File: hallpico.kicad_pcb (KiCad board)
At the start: 2 copper layers, 61 x 58.4 mm, 20 parts, among them J1 BOOT Jump Wire, SW1 SW_SPST, SW2 SW_SPST, U1 RP2040 MiniPico V1.1, U2 GH39FKSW, U3 GH39FKSW, U4 GH39FKSW, U5 GH39FKSW

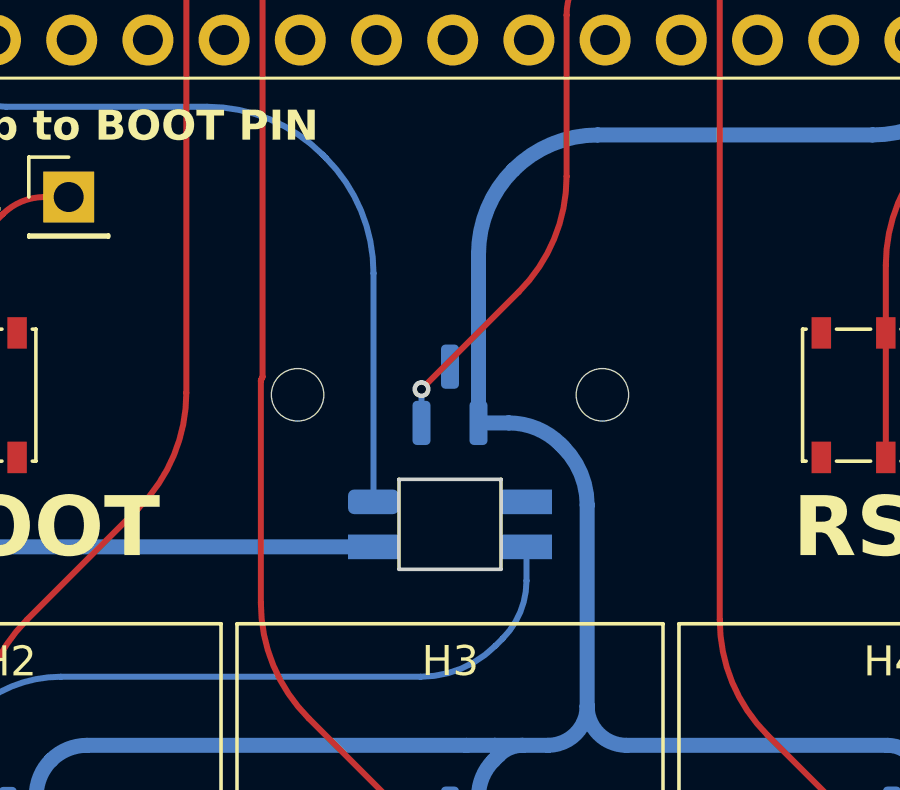
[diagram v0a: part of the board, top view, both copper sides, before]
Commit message: fix: update board with naming fix
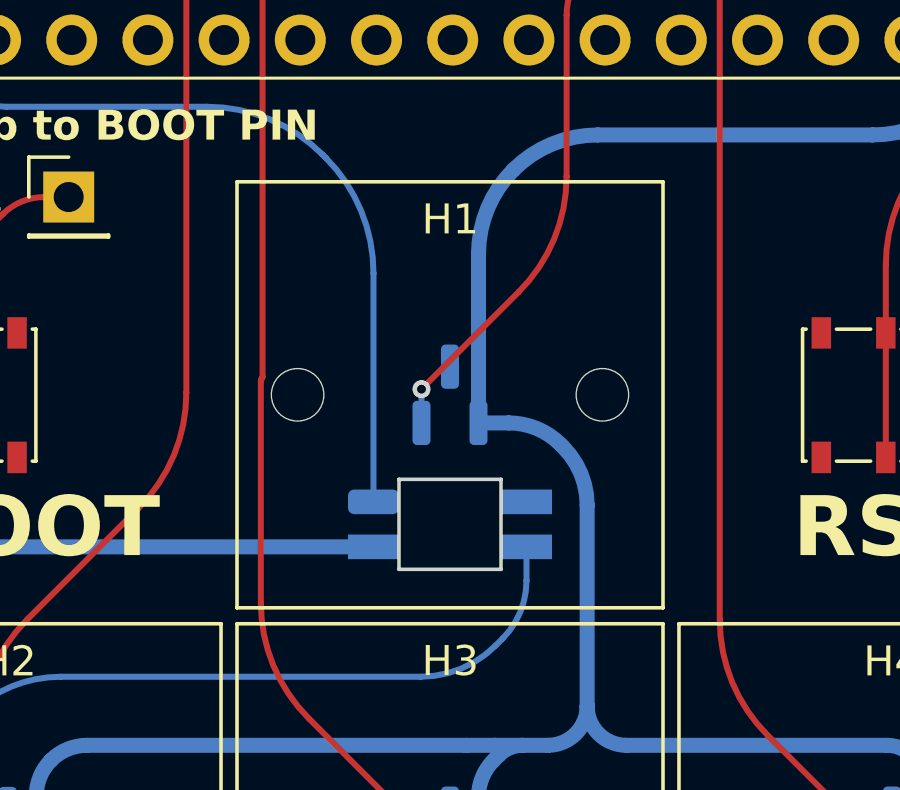
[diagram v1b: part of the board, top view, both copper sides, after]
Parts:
- H1: moved to F.Cu
- U1: value RP2040 MiniPico V1.1 -> RP2040 Pro Micro; footprint Library:RP2040_MiniPico_V1.1 -> Library:RP2040_ProMicro
- turned H1 to 0 degrees
